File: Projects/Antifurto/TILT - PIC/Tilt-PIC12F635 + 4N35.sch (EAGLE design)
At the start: 15 parts

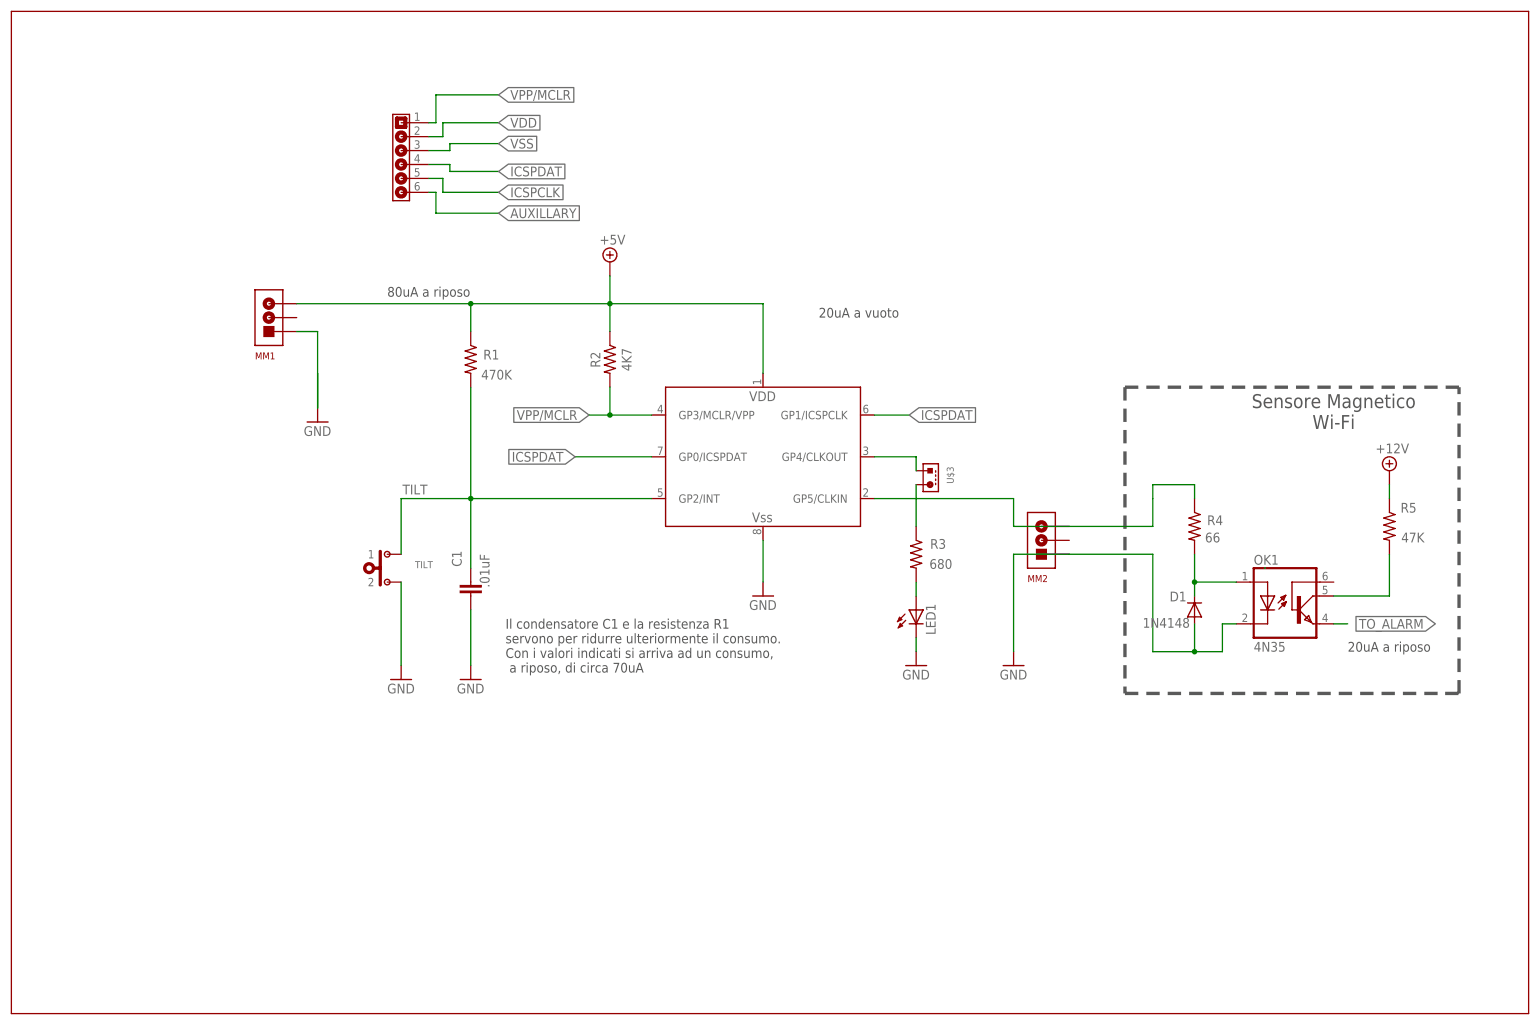
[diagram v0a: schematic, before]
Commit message: 2015-02-06 07:54 - commit with no comment
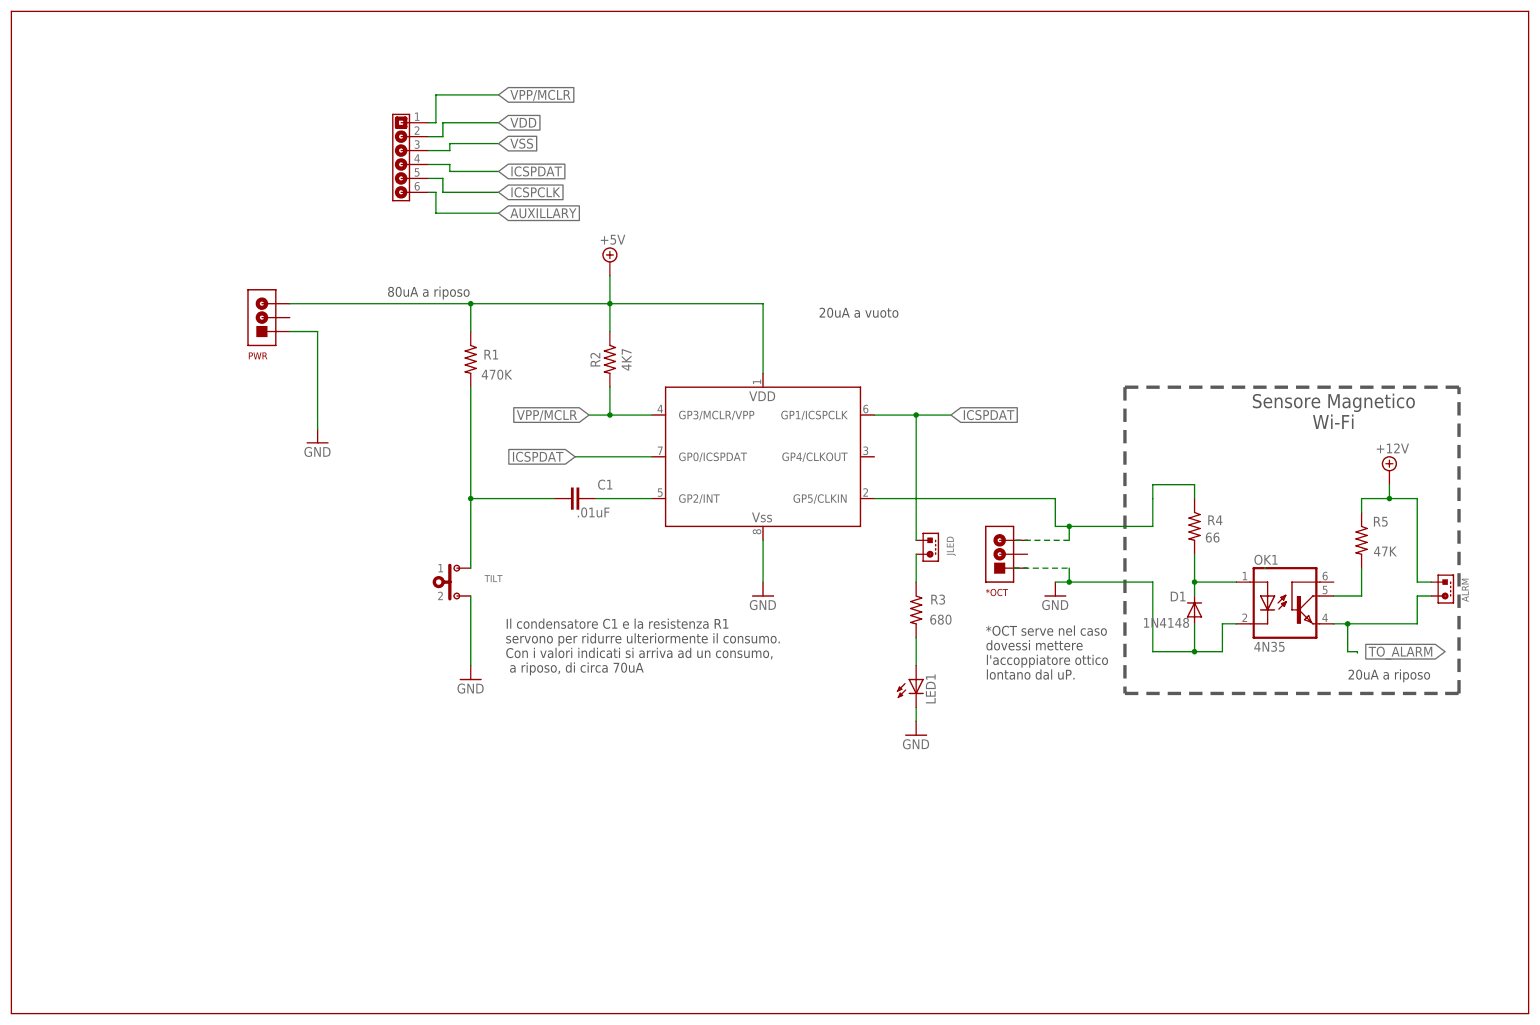
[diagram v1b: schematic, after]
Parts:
- removed MM1, MM2: MAMMUTH03, Ln-Varie:MAMMUTH03
- removed U$3: JUMPER2X1, Ln-Varie:JUMPER2X1
- added *OCT, PWR: MAMMUTH03, Ln-Varie:MAMMUTH03
- added ALRM, JLED: JUMPER2X1, Ln-Varie:JUMPER2X1
- renumbered U$2 to UP1
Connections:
- removed net N$5: U$3.1, UP1.GP4/CLKOUT
- new net N$4: C1.2, UP1.GP2/INT
- net +12V: now also ALRM.1
- net +5V: now also PWR.3
- net GND: now also PWR.1; no longer C1.1, MM2.1
- net ICSPDAT: now also JLED.1
- net N$3: no longer MM2.3
- net N$6: now also JLED.2; no longer U$3.2
- net TILT: now also C1.1; no longer UP1.GP2/INT
- net TO_ALARM: now also ALRM.2
- net VSS: no longer MM1.1
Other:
- note added: "*OCT serve nel caso dovessi mettere l'accoppiatore ottico lontano dal uP."
- moved on the sheet: C1, LED1, R3, R5, TILT
